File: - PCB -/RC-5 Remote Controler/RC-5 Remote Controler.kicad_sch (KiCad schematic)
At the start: 7 parts

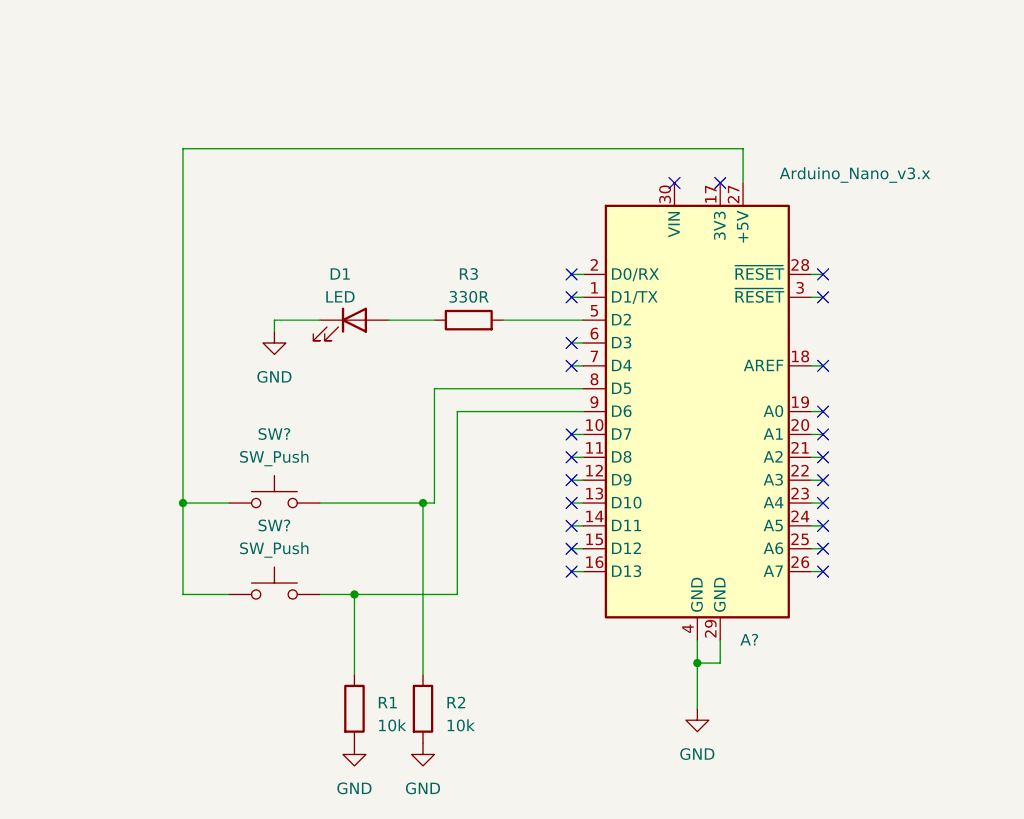
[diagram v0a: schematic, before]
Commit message: KICAD RC-5 PCB
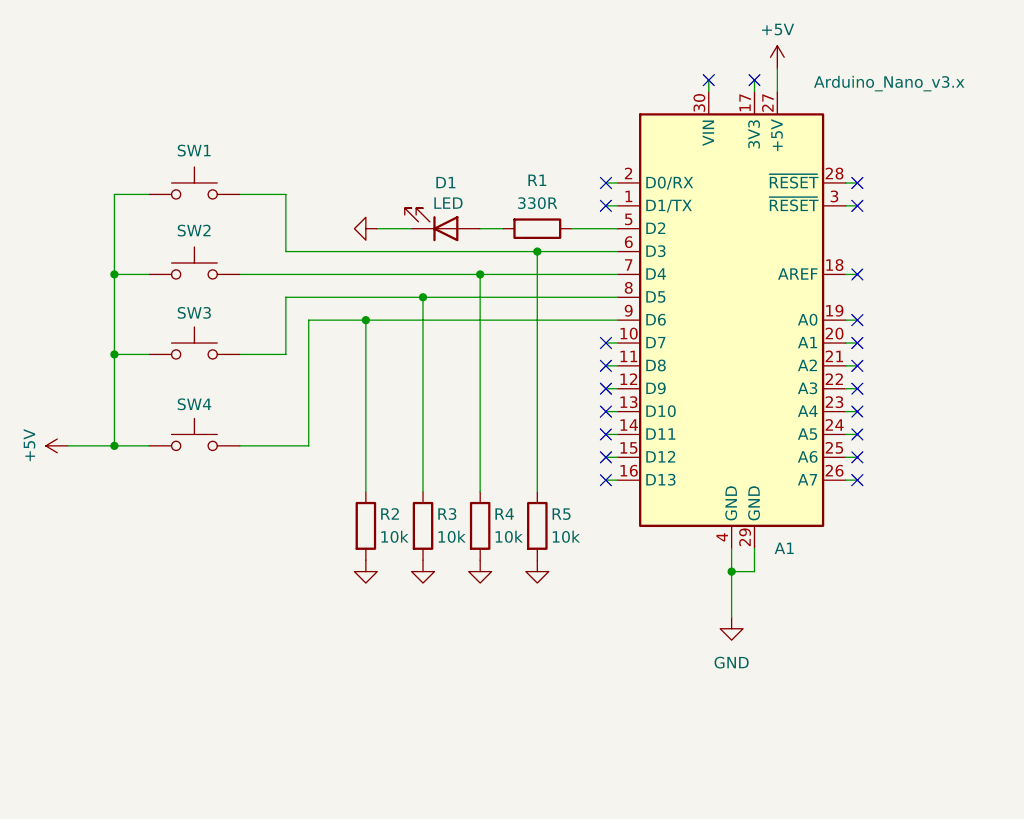
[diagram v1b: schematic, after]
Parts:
- removed A?: Arduino_Nano_v3.x, Module:Arduino_Nano, symbol MCU_Module:Arduino_Nano_v3.x
- removed SW? (x2): SW_Push, symbol Switch:SW_Push
- added A1: Arduino_Nano_v3.x, Module:Arduino_Nano, symbol MCU_Module:Arduino_Nano_v3.x
- added R4, R5: 10k, Resistor_THT:R_Axial_DIN0207_L6.3mm_D2.5mm_P10.16mm_Horizontal, symbol Device:R
- added SW1, SW2, SW3, SW4: SW_Push, Button_Switch_THT:SW_PUSH_6mm, symbol Switch:SW_Push
- D1: footprint (none) -> LED_THT:LED_D3.0mm_Horizontal_O3.81mm_Z6.0mm
- R1: value 10k -> 330R; footprint (none) -> Resistor_THT:R_Axial_DIN0207_L6.3mm_D2.5mm_P10.16mm_Horizontal
- R2: footprint (none) -> Resistor_THT:R_Axial_DIN0207_L6.3mm_D2.5mm_P10.16mm_Horizontal
- R3: value 330R -> 10k; footprint (none) -> Resistor_THT:R_Axial_DIN0207_L6.3mm_D2.5mm_P10.16mm_Horizontal
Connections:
- net GND: now also R3.2, A1.29 (GND), A1.4 (GND), R4.2, R5.2; no longer R1.2
- net at R1.1: now also A1.5 (D2)
- net at R2.1: now also A1.9 (D6), SW4.2
- net at R3.1: now also A1.8 (D5), SW3.2; no longer D1.2 (A)
- new net: A1.7 (D4), R4.1, SW2.2
- new net: D1.2 (A), R1.2
- new net: A1.6 (D3), R5.1, SW1.2
- new net +5V: A1.27 (+5V), SW1.1, SW2.1, SW3.1, SW4.1
- no-connect marks 24 -> 22
